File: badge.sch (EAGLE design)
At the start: 33 parts, among them IC1 MCP1703CB, U1 ESP8266, U2 AT25SF041-SOIC8, Y1 26MHz

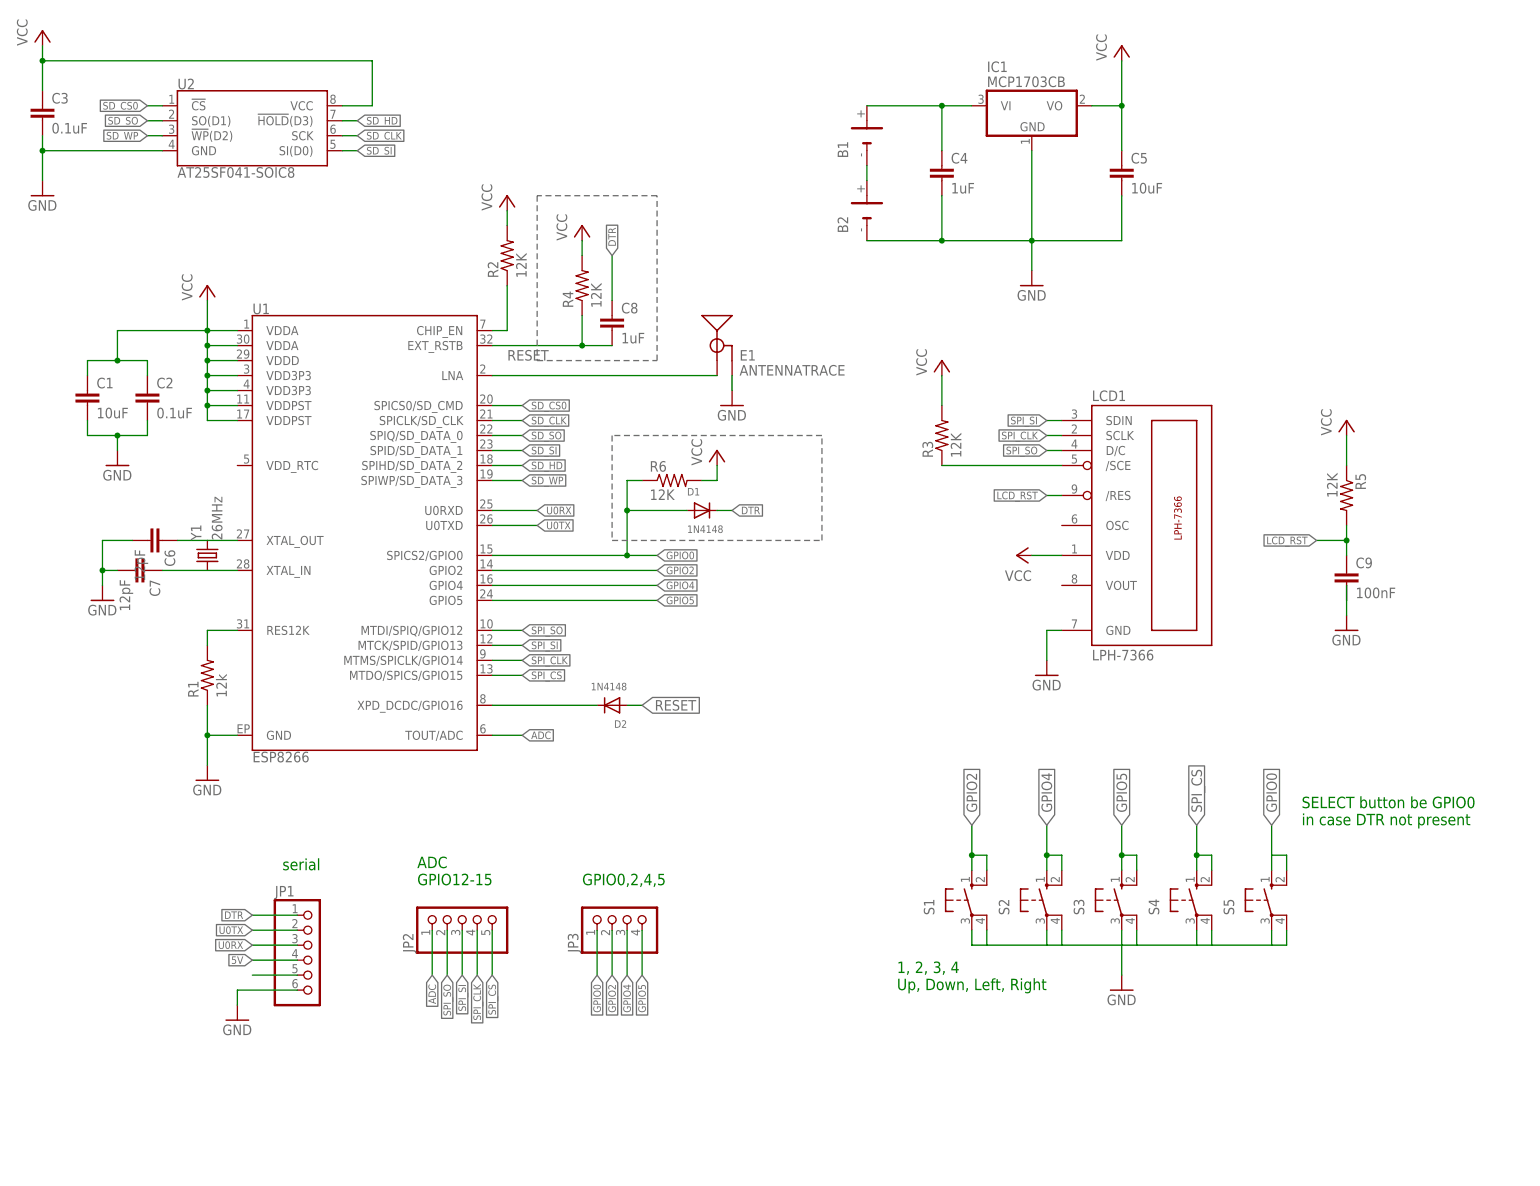
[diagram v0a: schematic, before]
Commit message: for ys
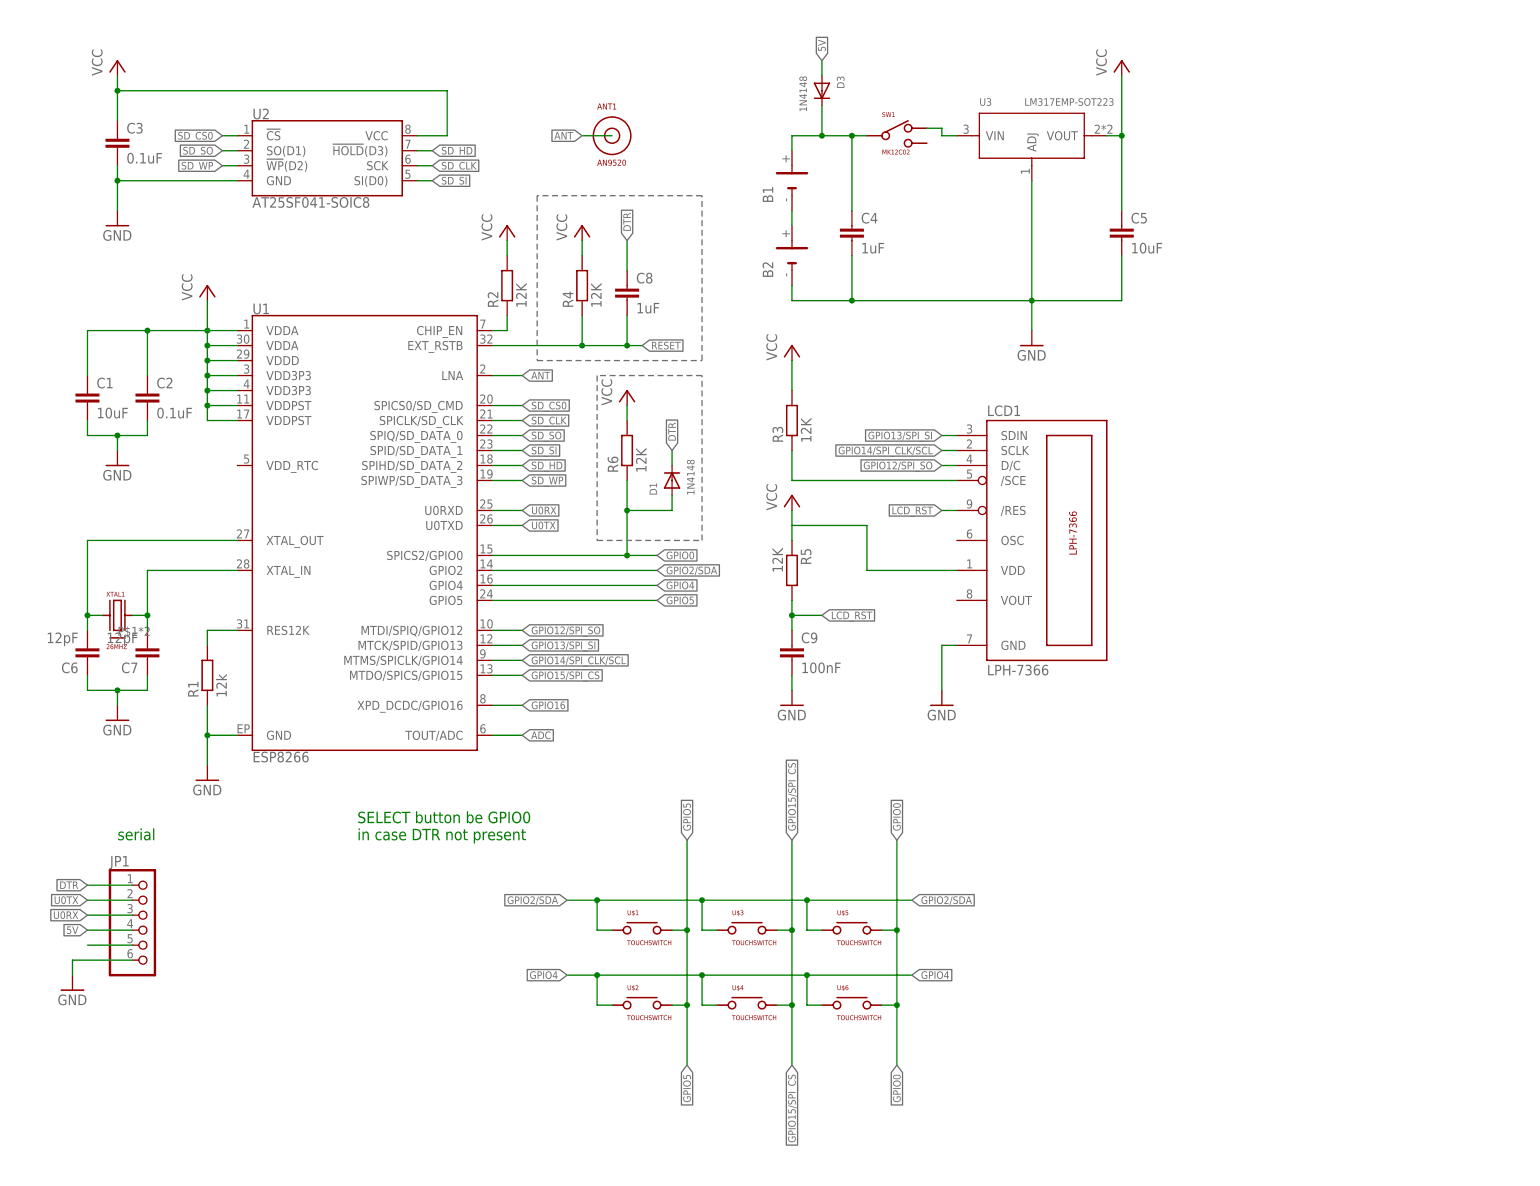
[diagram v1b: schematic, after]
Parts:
- removed D2: 1N4148, adafruit:DIODESOD-323F
- removed E1: ANTENNATRACE, SparkFun-RF:ANTENNATRACE
- removed IC1: MCP1703CB, linear:MCP1703CB
- removed JP2: (no value), pinhead:PINHD-1X5
- removed JP3: (no value), pinhead:PINHD-1X4
- removed S1, S2, S3, S4, S5: (no value), gm2:TACT-SW-4P-SMD
- removed Y1: 26MHz, SparkFun-FreqCtrl:CRYSTALCRYSTAL-SMD-5X3-16MHZ
- added ANT1: AN9520, badge:AN9520
- added D3: 1N4148, adafruit:DIODESOD-323F
- added SW1: MK12C02, badge:MK12C02
- added U$1, U$2, U$3, U$4, U$5, U$6: TOUCHSWITCH, badge:TOUCHSWITCH
- added U3: LM317EMP-SOT223, Seeed-OPL-ic:PMIC-LDO-LM317EMP(SOT223)
- added XTAL1: 26MHZ, badge:26MHZ
- C1, C2, C3, C4, C5, C6, C7, C8, C9: device rcl:C-EUC0805 -> resistor:C-EUC0603K
- R1, R2, R3, R4, R5, R6: device rcl:R-US_R0805 -> resistor:R-EU_R0603W
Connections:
- removed net GPIO2: JP3.2, S1.S, S1.S1, U1.GPIO2
- removed net N$7: C7.1, U1.XTAL_IN, Y1.1
- removed net SPI_CLK: JP2.4, LCD1.SCLK, U1.MTMS/SPICLK/GPIO14
- removed net SPI_CS: JP2.5, S4.S, S4.S1, U1.MTDO/SPICS/GPIO15
- removed net SPI_SI: JP2.3, LCD1.SDIN, U1.MTCK/SPID/GPIO13
- removed net SPI_SO: JP2.2, LCD1.D/C, U1.MTDI/SPIQ/GPIO12
- new net ANT: ANT1.P$1, U1.LNA
- new net GPIO12/SPI_SO: LCD1.D/C, U1.MTDI/SPIQ/GPIO12
- new net GPIO13/SPI_SI: LCD1.SDIN, U1.MTCK/SPID/GPIO13
- new net GPIO14/SPI_CLK/SCL: LCD1.SCLK, U1.MTMS/SPICLK/GPIO14
- new net GPIO15/SPI_CS: U$3.P$2, U$4.P$2, U1.MTDO/SPICS/GPIO15
- new net GPIO16: U1.XPD_DCDC/GPIO16
- new net GPIO2/SDA: U$1.P$1, U$3.P$1, U$5.P$1, U1.GPIO2
- net 5V: now also D3.A
- net ADC: no longer JP2.1
- net GND: now also C6.1, C7.1, U3.ADJ; no longer C6.2, C7.2, E1.GND, IC1.GND, S1.P, S1.P1, S2.P, S2.P1, S3.P, S3.P1, S4.P, S4.P1, S5.P, S5.P1
- net GPIO0: now also U$5.P$2, U$6.P$2; no longer JP3.1, S5.S, S5.S1
- net GPIO4: now also U$2.P$1, U$4.P$1, U$6.P$1; no longer JP3.3, S2.S, S2.S1
- net GPIO5: now also U$1.P$2, U$2.P$2; no longer JP3.4, S3.S, S3.S1
- net N$1: now also SW1.P$2, U3.VIN; no longer E1.SIGNAL, U1.LNA
- net N$5: now also D3.C, SW1.P$1; no longer IC1.VI
- net N$6: now also C6.2, U1.XTAL_OUT, XTAL1.P$1; no longer D2.C, U1.XPD_DCDC/GPIO16
- net N$8: now also C7.2, U1.XTAL_IN, XTAL1.P$2; no longer C6.1, U1.XTAL_OUT, Y1.2
- net RESET: no longer D2.A
- net VCC: now also U3.VOUT; no longer IC1.VO
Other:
- note removed: "1, 2, 3, 4 Up, Down, Left, Right"
- note removed: "ADC GPIO12-15"
- note removed: "GPIO0,2,4,5"
- moved on the sheet: B1, B2, C3, C4, C5, C6, C7, C8, C9, D1, JP1, LCD1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
